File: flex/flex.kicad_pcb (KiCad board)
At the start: 2 copper layers, 104.1 x 90.6 mm, 105 parts, among them J1 Conn_01x04_Female, J2 Conn_01x05_Female, J3 Conn_01x03_Female, J4 Conn_01x06_Female, J5 Conn_01x03_Female, SW10 NA_SW_Push, SW11 NA_SW_Push, SW12 NA_SW_Push, SW15 NA_SW_Push, SW16 NA_SW_Push, SW17 NA_SW_Push, SW20 NA_SW_Push, SW21 NA_SW_Push, SW22 NA_SW_Push, SW24 NA_SW_Push, SW25 NA_SW_Push, SW26 NA_SW_Push, SW6 NA_SW_Push, SW7 NA_SW_Push, SW8 NA_SW_Push

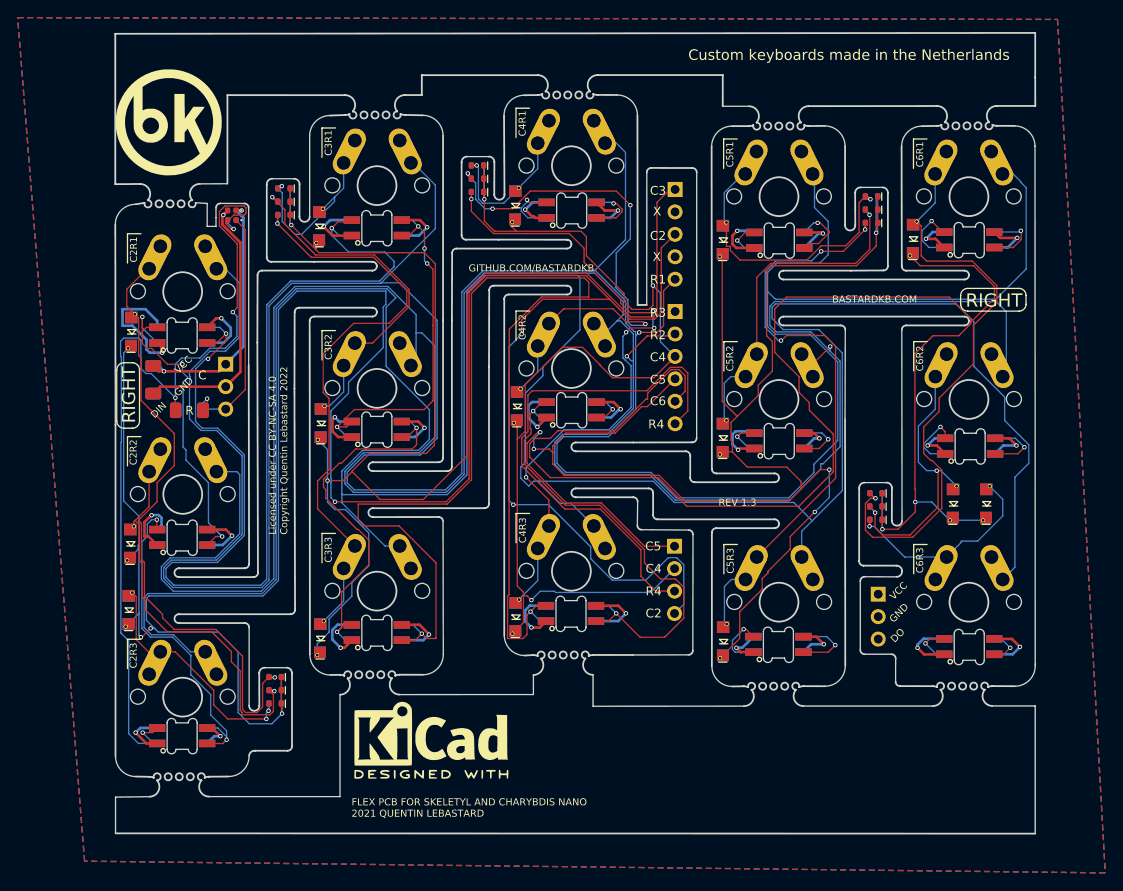
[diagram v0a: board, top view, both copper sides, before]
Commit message: routing
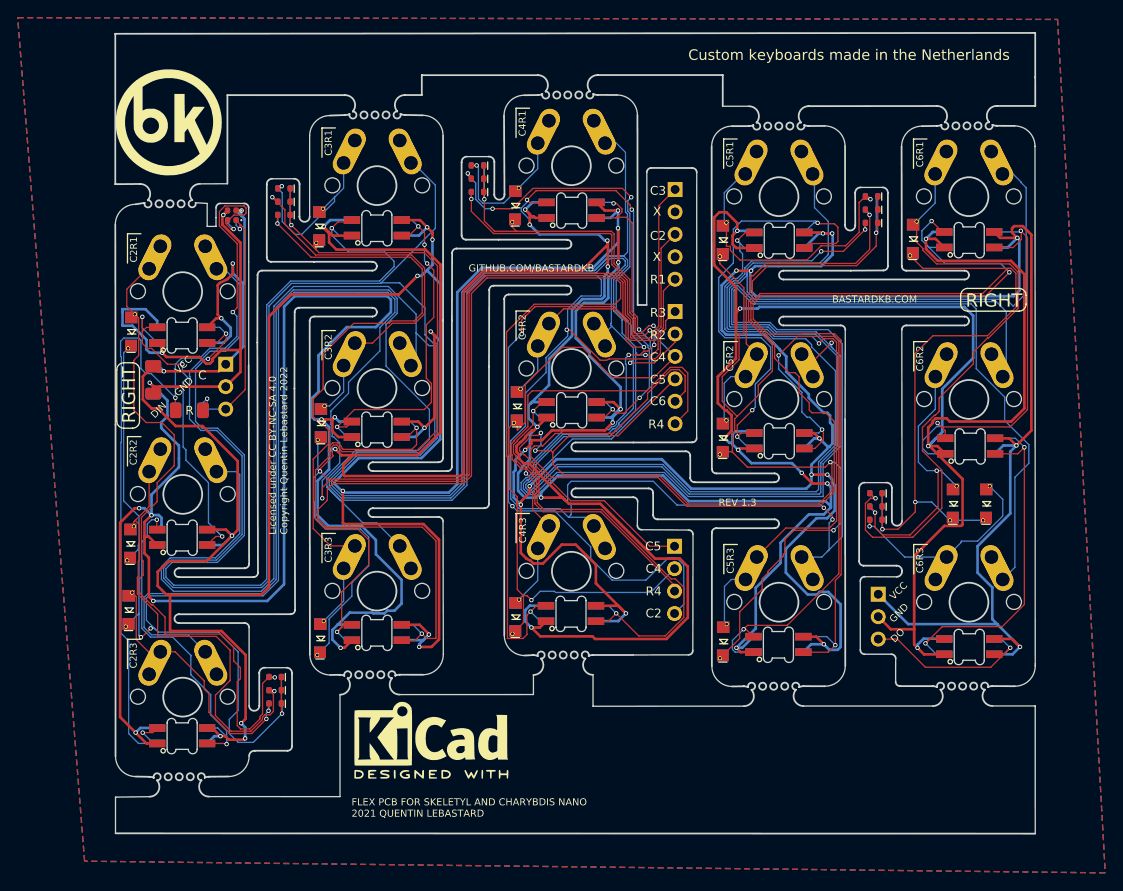
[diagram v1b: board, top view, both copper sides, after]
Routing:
- net Gnd: track 131.8 -> 750.0 mm, vias 16 -> 29
- net Vcc: track 118.0 -> 700.7 mm, vias 17 -> 36
- net Net-(D41-DOUT): track 11.3 -> 128.8 mm, vias 2 -> 3
- net Net-(D51-DOUT): track 15.4 -> 104.1 mm, vias 2 -> 3
- net Net-(D49-DOUT): track 12.9 -> 71.1 mm, vias 2 -> 3
- net row4: track 326.3 -> 378.6 mm, vias 0 -> 3
- net Net-(D47-DOUT): track 11.9 -> 55.4 mm, vias 2 -> 3
- net Net-(D39-DOUT): track 11.5 -> 51.4 mm, vias 2 -> 4
- net row2: track 390.3 -> 429.6 mm
- net Net-(D55-DOUT): track 14.8 -> 48.0 mm
- net row3: track 307.3 -> 338.8 mm
- net Net-(D57-DOUT): track 12.3 -> 43.2 mm
- net Net-(D25-DOUT): track 134.2 -> 152.1 mm
- net Dout: track 4.37 -> 21.5 mm
- net col2: track 297.4 -> 314.5 mm
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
